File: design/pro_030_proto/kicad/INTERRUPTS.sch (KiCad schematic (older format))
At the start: 11 parts, among them IC28 74LS148

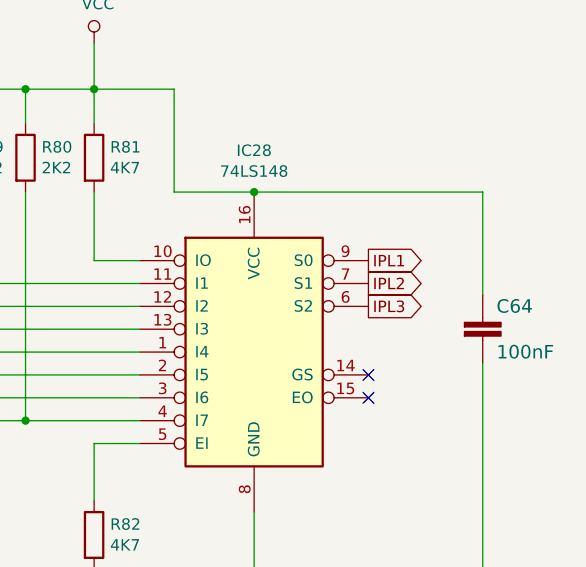
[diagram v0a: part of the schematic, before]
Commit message: Finally fix ERC...
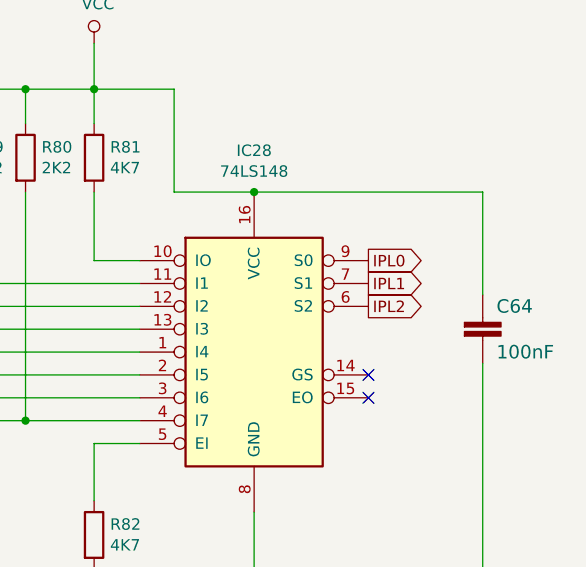
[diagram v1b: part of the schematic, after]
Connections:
- net IPL3 is gone; now on net IPL2: IC28.6 (S2)
- net IPL1: now also IC28.7 (S1); no longer IC28.9 (S0)
- net IPL2: no longer IC28.7 (S1)
- new net IPL0: IC28.9 (S0)
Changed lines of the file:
@@
 Connection ~ 6450 2750
 Text GLabel 7650 3700 2    50   Output ~ 0
-IPL3
+IPL2
 Text GLabel 7650 3600 2    50   Output ~ 0
-IPL2
+IPL1
 Text GLabel 7650 3500 2    50   Output ~ 0
-IPL1
+IPL0
 Connection ~ 7150 4900
 Wire Wire Line
